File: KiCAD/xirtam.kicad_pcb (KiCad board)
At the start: 2 copper layers, 71.1 x 51.8 mm, 25 parts, among them J1 Conn_01x15_Female, J2 Conn_01x15_Male, J3 Power, J4 JTAG, J5 Bootloader, P1 USB_A, SW1 SW_Push_SPDT, U1 MT093APR1, U2 AT90USB1287, Y1 16 MHz Crystal

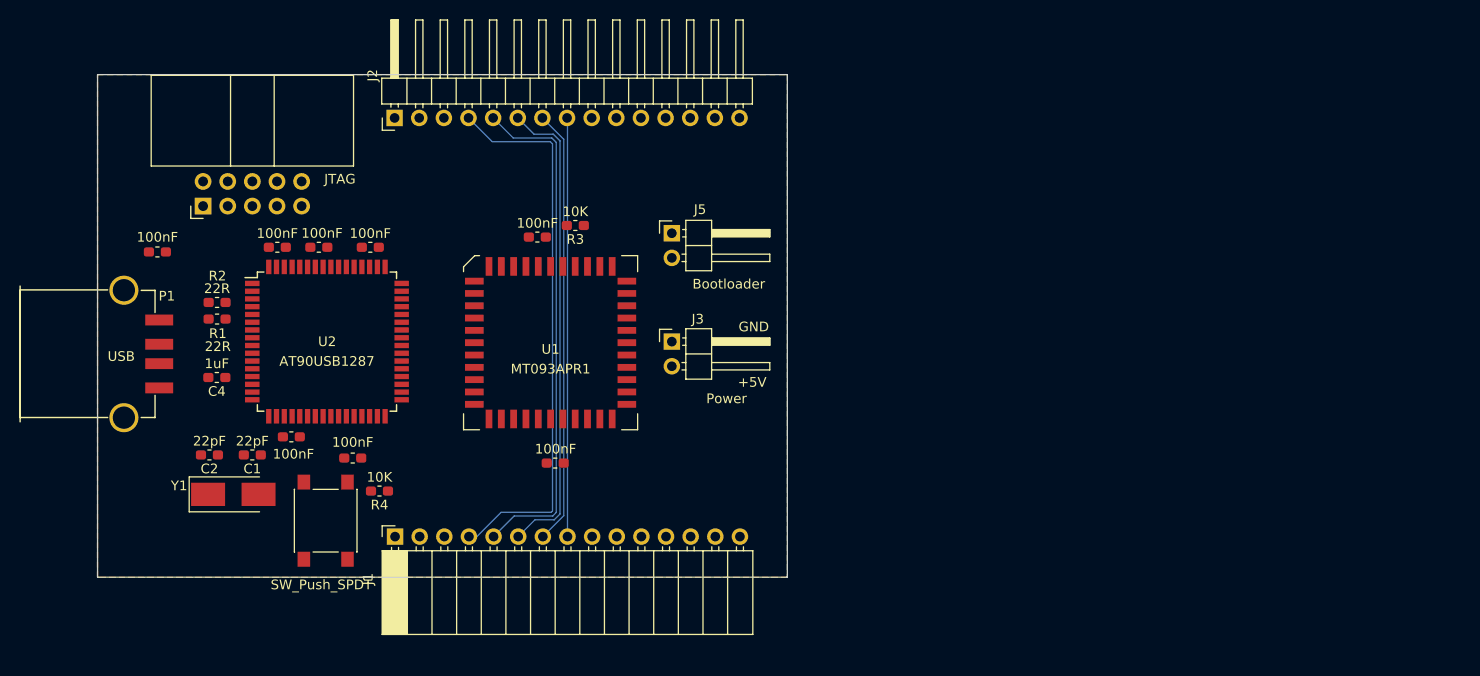
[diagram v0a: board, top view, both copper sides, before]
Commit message: New PCB layout
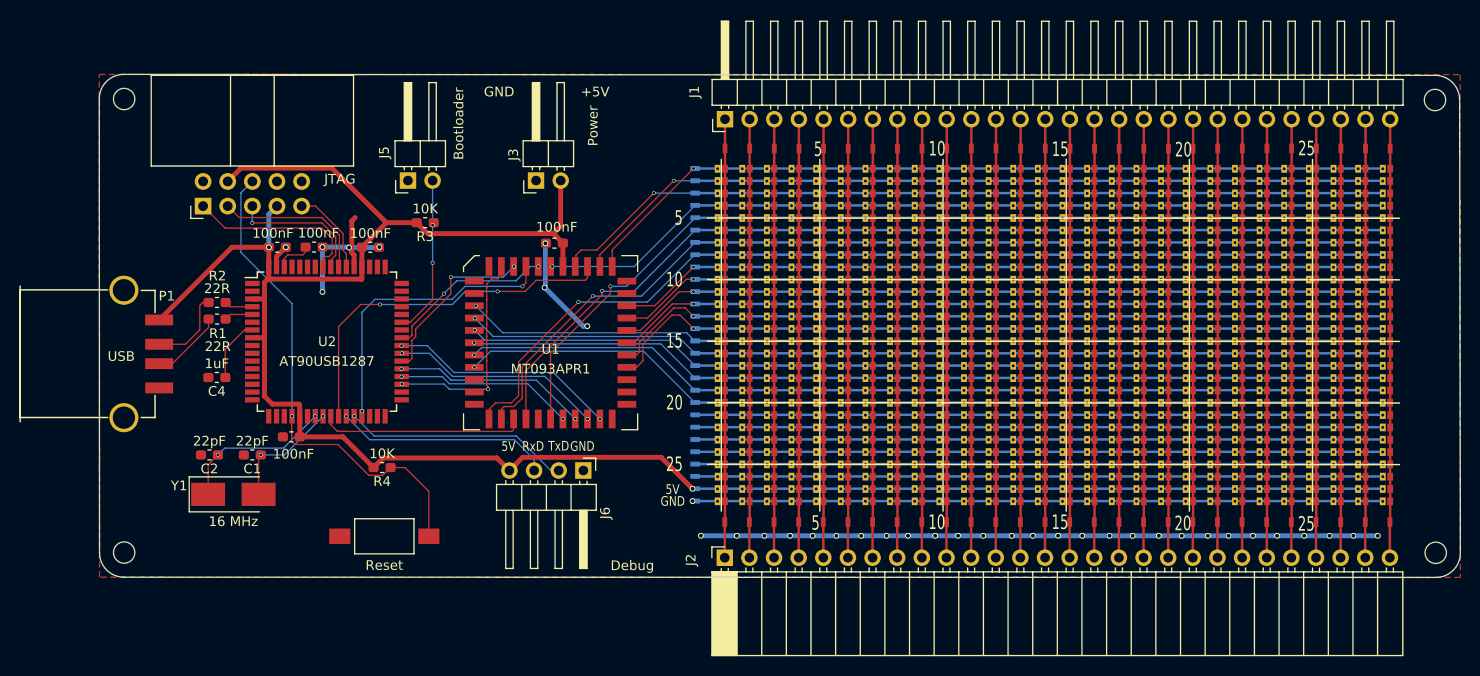
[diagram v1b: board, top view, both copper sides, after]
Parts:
- removed the C7 at (167.8, 120.3)
- removed the C8 at (147.0, 119.8)
- removed C9: 100nF, Capacitor_SMD:C_0603_1608Metric_Pad1.05x0.95mm_HandSolder
- added J6: Debug, Connector_PinHeader_2.54mm:PinHeader_1x04_P2.54mm_Horizontal, F.Cu at (170.7, 121.1)
- added M1: MatrixInterconnectMatrix, Jumper:matrixinterconnectmatrix, F.Cu at (182.0, 88.6)
- added REF**: MountingHole_2.2mm_M2, MountingHole:MountingHole_2.2mm_M2, F.Cu at (123.4, 82.8)
- added REF**: MountingHole_2.2mm_M2, MountingHole:MountingHole_2.2mm_M2, F.Cu at (123.4, 129.5)
- added REF**: MountingHole_2.2mm_M2, MountingHole:MountingHole_2.2mm_M2, F.Cu at (258.6, 129.6)
- added REF**: MountingHole_2.2mm_M2, MountingHole:MountingHole_2.2mm_M2, F.Cu at (258.5, 82.9)
- J1: value Conn_01x15_Female -> Conn_01x28_Male; footprint Connector_PinSocket_2.54mm:PinSocket_1x15_P2.54mm_Horizontal -> Connector_PinHeader_2.54mm:PinHeader_1x28_P2.54mm_Horizontal
- J2: value Conn_01x15_Male -> Conn_01x28_Female; footprint Connector_PinHeader_2.54mm:PinHeader_1x15_P2.54mm_Horizontal -> Connector_PinSocket_2.54mm:PinSocket_1x28_P2.54mm_Horizontal
- SW1: value SW_Push_SPDT -> Reset; footprint Button_Switch_SMD:SW_Push_1P1T_NO_6x6mm_H9.5mm -> Button_Switch_SMD:SW_SPST_FSMSM
- Y1: value 16 MHz Crystal -> 16 MHz
- moved J2 56.7 mm to (185.3, 130.1)
- moved J1 54.9 mm to (185.3, 84.9)
- moved J5 27.7 mm to (152.7, 91.2), turned to 90 degrees
- moved J3 21.7 mm to (165.9, 91.2), turned to 90 degrees
- moved R3 15.5 mm to (154.4, 95.5)
- moved SW1 6.26 mm to (150.2, 127.9), turned to 0 degrees
- moved R4 2.44 mm to (150.0, 120.8)
- moved C8 1.87 mm to (167.8, 97.6), turned to 0 degrees
- moved C3 0.49 mm to (143.0, 98.0)
- renumbered C10 to C7, C11 to C8
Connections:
- J2 pad 1: Net-(J1-Pad1) -> Net-(J2-Pad1)
- J2 pad 10: Net-(J1-Pad10) -> Net-(J2-Pad10)
- J2 pad 11: Net-(J1-Pad11) -> Net-(J2-Pad11)
- J2 pad 12: Net-(J1-Pad12) -> Net-(J2-Pad12)
- J2 pad 13: Net-(J1-Pad13) -> Net-(J2-Pad13)
- J2 pad 14: Net-(J1-Pad14) -> Net-(J2-Pad14)
- J2 pad 15: Net-(J1-Pad15) -> Net-(J2-Pad15)
- J2 pad 2: Net-(J1-Pad2) -> Net-(J2-Pad2)
- J2 pad 3: Net-(J1-Pad3) -> Net-(J2-Pad3)
- J2 pad 4: Net-(J1-Pad4) -> Net-(J2-Pad4)
- J2 pad 5: Net-(J1-Pad5) -> Net-(J2-Pad5)
- J2 pad 6: Net-(J1-Pad6) -> Net-(J2-Pad6)
- J2 pad 7: Net-(J1-Pad7) -> Net-(J2-Pad7)
- J2 pad 8: Net-(J1-Pad8) -> Net-(J2-Pad8)
- J2 pad 9: Net-(J1-Pad9) -> Net-(J2-Pad9)
- SW1 pad 1: ~RESET -> GND
- SW1 pad 2: GND -> ~RESET
- U1 pad 1: Net-(J1-Pad1) -> Net-(M1-Pad4)
- U1 pad 10: (no net) -> Net-(M1-Pad16)
- U1 pad 11: (no net) -> Net-(M1-Pad17)
- U1 pad 12: (no net) -> Net-(M1-Pad18)
- U1 pad 13: (no net) -> Net-(M1-Pad19)
- U1 pad 14: (no net) -> Net-(M1-Pad20)
- U1 pad 18: Net-(J1-Pad2) -> Net-(M1-Pad8)
- U1 pad 19: Net-(J1-Pad3) -> Net-(M1-Pad7)
- U1 pad 21: Net-(J1-Pad4) -> Net-(M1-Pad6)
- U1 pad 23: Net-(J1-Pad5) -> Net-(M1-Pad5)
- U1 pad 32: Net-(J1-Pad8) -> Net-(M1-Pad14)
- U1 pad 33: Net-(J1-Pad9) -> Net-(M1-Pad13)
- U1 pad 34: Net-(J1-Pad12) -> Net-(M1-Pad12)
- U1 pad 35: Net-(J1-Pad13) -> Net-(M1-Pad11)
- U1 pad 36: Net-(J1-Pad14) -> Net-(M1-Pad10)
- U1 pad 37: Net-(J1-Pad15) -> Net-(M1-Pad9)
- U1 pad 40: Net-(J1-Pad7) -> Net-(M1-Pad1)
- U1 pad 41: Net-(J1-Pad10) -> Net-(M1-Pad2)
- U1 pad 43: Net-(J1-Pad11) -> Net-(M1-Pad3)
- U1 pad 9: Net-(J1-Pad6) -> Net-(M1-Pad15)
- U2 pad 10: Net-(U1-Pad3) -> (no net)
- U2 pad 11: Net-(U1-Pad20) -> (no net)
- U2 pad 25: (no net) -> Net-(U1-Pad20)
- U2 pad 26: (no net) -> Net-(U1-Pad42)
- U2 pad 27: (no net) -> /RxD
- U2 pad 28: (no net) -> /TxD
- U2 pad 29: (no net) -> Net-(U1-Pad3)
- U2 pad 35: Net-(U1-Pad42) -> Net-(U1-Pad5)
- U2 pad 36: Net-(U1-Pad5) -> Net-(U1-Pad24)
- U2 pad 37: Net-(U1-Pad24) -> Net-(U1-Pad25)
- U2 pad 38: Net-(U1-Pad25) -> Net-(U1-Pad4)
- U2 pad 39: Net-(U1-Pad4) -> Net-(U1-Pad26)
- U2 pad 40: Net-(U1-Pad26) -> Net-(U1-Pad27)
- U2 pad 41: Net-(U1-Pad27) -> Net-(U1-Pad2)
- U2 pad 42: Net-(U1-Pad2) -> (no net)
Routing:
- net +5V: track 0.00 -> 152.4 mm, vias 0 -> 2
- net GND: track 0.00 -> 99.3 mm, vias 0 -> 37
- net Net-(J1-Pad4): track 57.3 -> 3.02 mm
- net ~RESET: track 0.00 -> 51.1 mm, vias 0 -> 1
- net Net-(J1-Pad5): track 53.2 -> 3.02 mm
- net Net-(J1-Pad6): track 49.1 -> 3.02 mm
- net Net-(J1-Pad7): track 45.0 -> 3.02 mm
- net Net-(J1-Pad8): track 43.2 -> 3.02 mm
- net Net-(U1-Pad42): track 0.00 -> 38.2 mm, vias 0 -> 2
- net Net-(M1-Pad8): track 0.00 -> 30.9 mm, vias 0 -> 1
- net Net-(U1-Pad3): track 0.00 -> 30.1 mm, vias 0 -> 2
- net Net-(M1-Pad7): track 0.00 -> 29.9 mm, vias 0 -> 1
- net Net-(M1-Pad6): track 0.00 -> 28.6 mm, vias 0 -> 1
- net Net-(M1-Pad5): track 0.00 -> 27.8 mm, vias 0 -> 1
- net Net-(M1-Pad20): track 0.00 -> 25.6 mm, vias 0 -> 1
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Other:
- board size 71.1 x 51.8 mm -> 140.3 x 51.9 mm
- board text added: "10"
- board text added: "15"
- board text added: "20"
- board text added: "25"
- board text added: "5"
- board text added: "5V"
- board text added: "RxD"
- board text added: "TxD"
